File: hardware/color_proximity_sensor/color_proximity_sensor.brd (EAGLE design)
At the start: 48 x 25 mm, 65 parts, among them IC1 TCS37725FN, IC2 APDS-9800-021, IC4 LM25011MY, IC5 ATXMEGA64DA-AU, J1 PDI_ATMEL_WIDTH, Q1 16 MHz, T1 BC847CDXV6T1G, T4 BC847CDXV6T1G

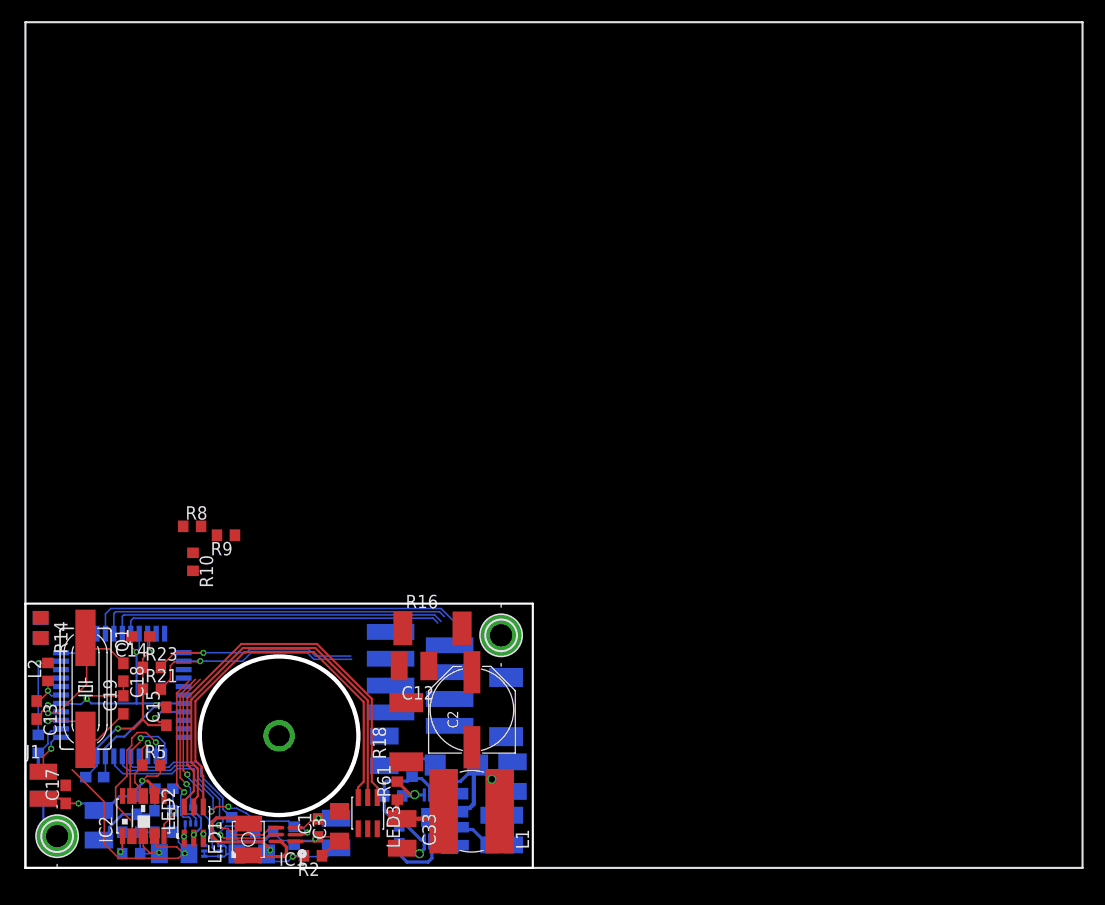
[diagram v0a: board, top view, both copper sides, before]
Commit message: board routed
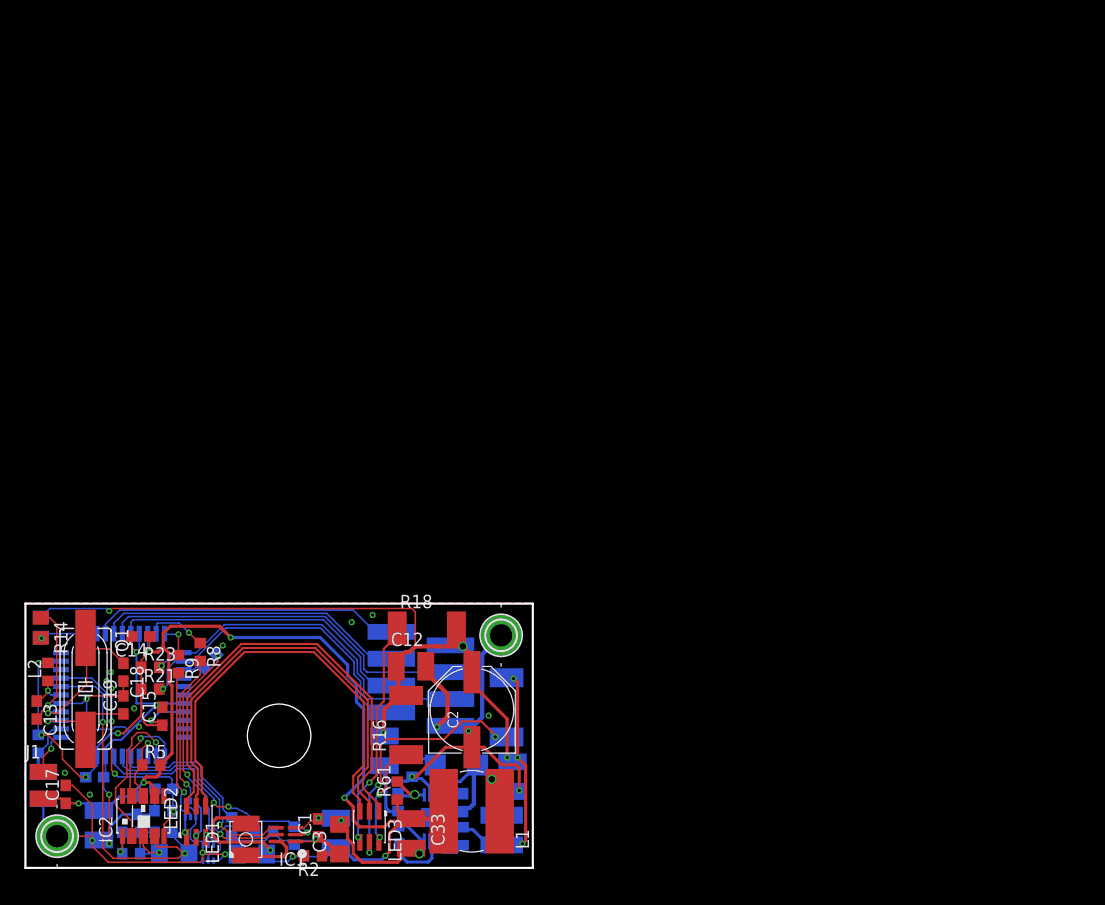
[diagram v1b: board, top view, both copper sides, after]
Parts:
- moved R9 13.0 mm to (14.5, 19.3), turned to 270 degrees
- moved R8 11.9 mm to (16.5, 20.4), turned to 270 degrees
- moved R18 10.0 mm to (38.0, 22.7), turned to 0 degrees
- moved R10 9.51 mm to (17.4, 19.6), flipped to the bottom, turned to 135 degrees
- moved R16 9.48 mm to (36.0, 13.5), turned to 90 degrees
- moved LED3 1.30 mm to (32.5, 3.89)
- moved C3 1.22 mm to (29.7, 2.72)
- moved C33 0.84 mm to (36.5, 3.26)
- moved R60 0.74 mm to (35.3, 6.22), turned to 270 degrees
- moved T4 0.61 mm to (15.6, 5.56)
- moved T1 0.41 mm to (17.3, 1.45), turned to 0 degrees
- moved C15 0.38 mm to (13.0, 14.4)
- moved C12 0.28 mm to (36.5, 19.1), turned to 0 degrees
- moved LED2 0.24 mm to (16.2, 4.37)
- moved LED1 0.23 mm to (20.9, 2.69)
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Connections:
- net +24V: now also COM.7; no longer COM.8
- net APDS_AMBIENT_0-300MV: now also IC5.40; no longer IC5.1
- net APDS_PROXIMITY_ANA_0-0.65V: now also IC5.41; no longer IC5.44
- net BATTERY_MONITOR_0-1V: now also IC5.1; no longer IC5.40
- net COLOR_DATA0_3V3: now also COM.6; no longer COM.3
- net COLOR_DATA1_3V3: now also COM.5; no longer COM.2
- net COLOR_DATA2_3V3: now also COM.4; no longer COM.1
- net COLOR_VALID_OUT_3V3: now also COM.8; no longer COM.4
- net GND: now also COM.1; no longer COM.5
- net LED_GREEN_CMD_3V3: now also IC5.11; no longer IC5.14
- net LED_RED_CMD_3V3: now also IC5.14; no longer IC5.11
- net RX_3V3: now also COM.3; no longer COM.6
- net TX_3V3: now also COM.2; no longer COM.7
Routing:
- net GND: track 92.5 -> 195.9 mm, vias 7 -> 28
- net +24V: track 7.66 -> 98.7 mm, vias 0 -> 7
- net +3V3: track 80.7 -> 153.3 mm, vias 8 -> 13
- net N$11: track 0.00 -> 26.3 mm, vias 0 -> 3
- net N$6: track 0.00 -> 22.4 mm, vias 0 -> 2
- net APDS_PROXIMITY_ANA_0-0.65V: track 7.10 -> 25.0 mm, vias 1 -> 3
- net RX_3V3: track 22.7 -> 34.1 mm
- net APDS_AMBIENT_0-300MV: track 23.6 -> 34.2 mm, vias 1 -> 2
- net N$12: track 0.00 -> 10.6 mm, vias 0 -> 2
- net TX_3V3: track 22.1 -> 30.3 mm
- net BATTERY_MONITOR_0-1V: track 0.00 -> 7.54 mm, vias 0 -> 1
- net COLOR_VALID_OUT_3V3: track 35.3 -> 29.3 mm
- net LED_BLUE_CMD_3V3: track 0.00 -> 5.97 mm, vias 0 -> 1
- net N$5: track 18.6 -> 23.4 mm, vias 1 -> 2
- net COLOR_DATA0_3V3: track 33.4 -> 29.4 mm
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- added copper zone on layer 1, net GND
- added copper zone on layer 16, net GND
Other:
- outline, holes or cut-outs redrawn
